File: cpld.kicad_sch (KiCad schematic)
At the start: 1 part, among them U6 ATF1508AS-10AU100

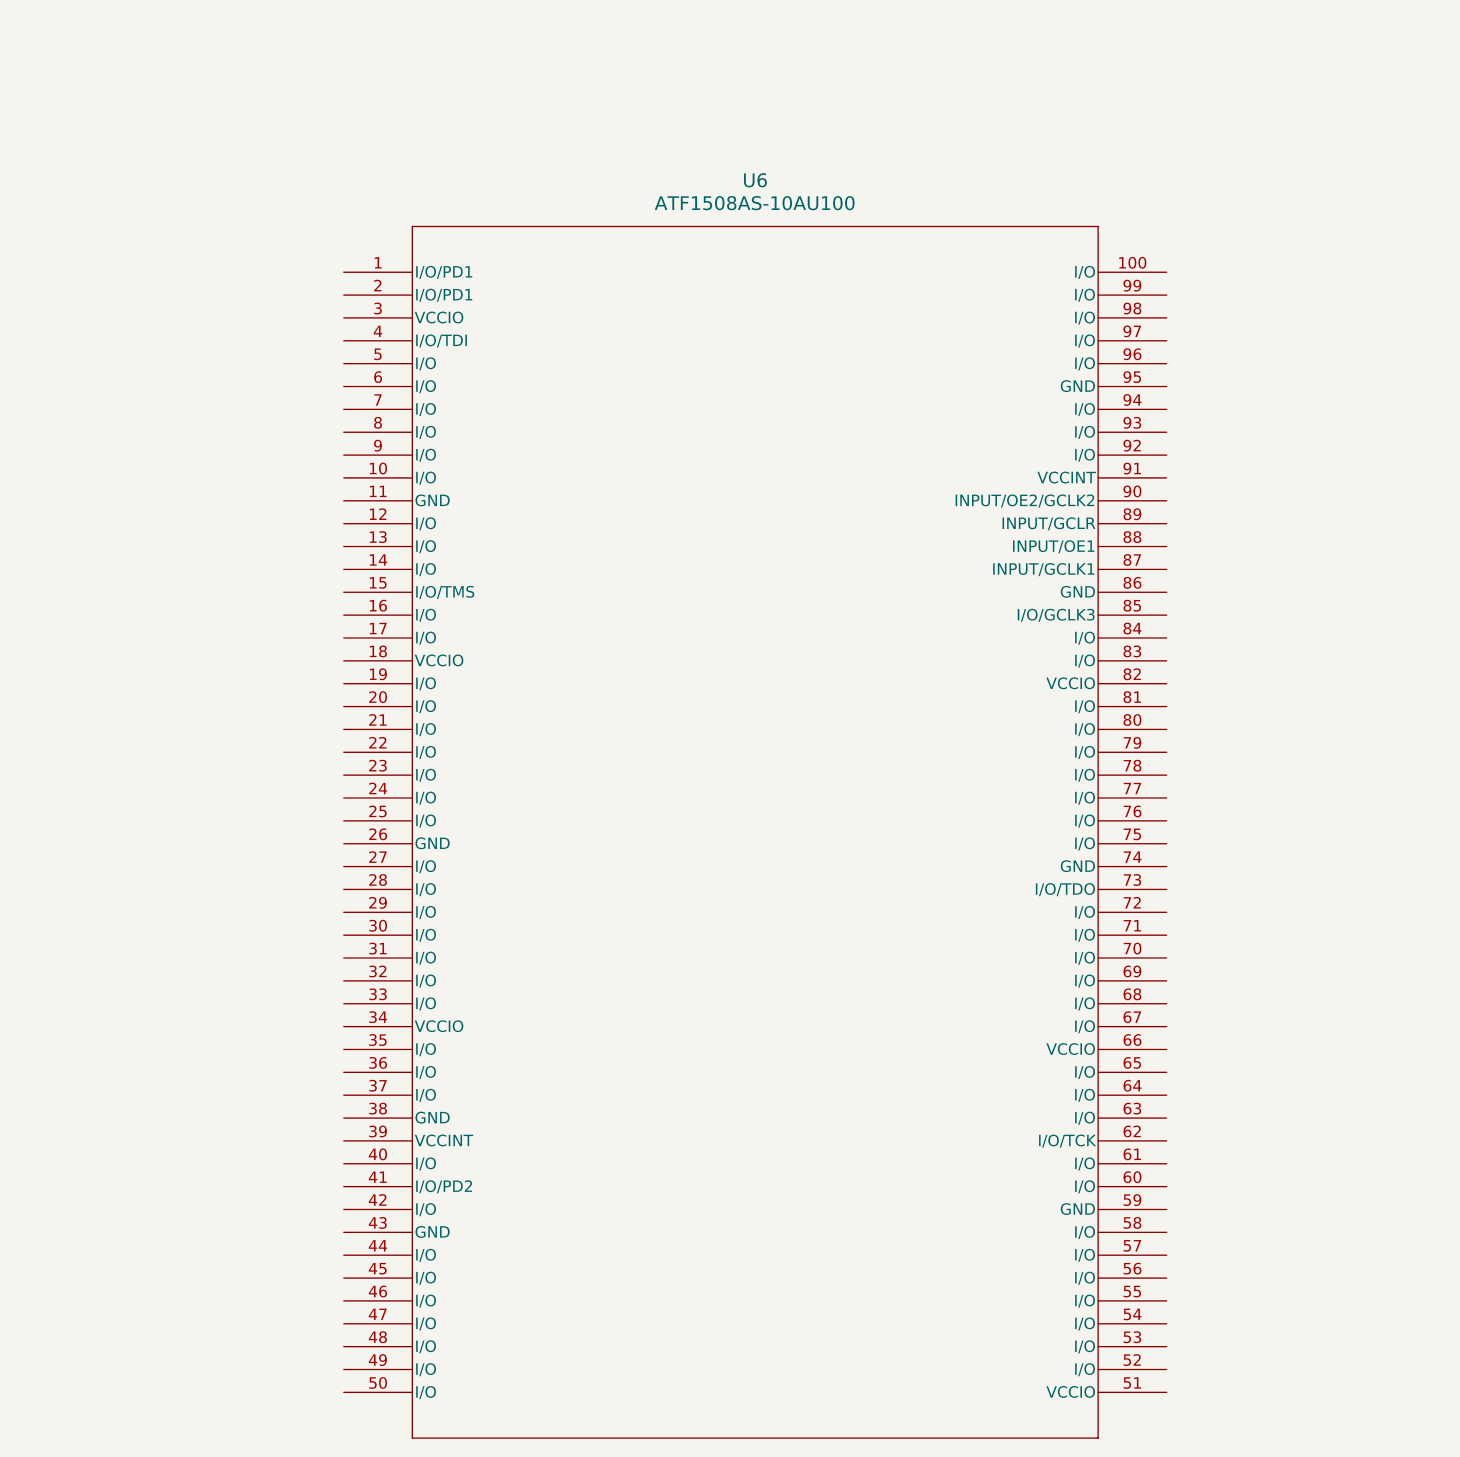
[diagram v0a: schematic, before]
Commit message: Update design
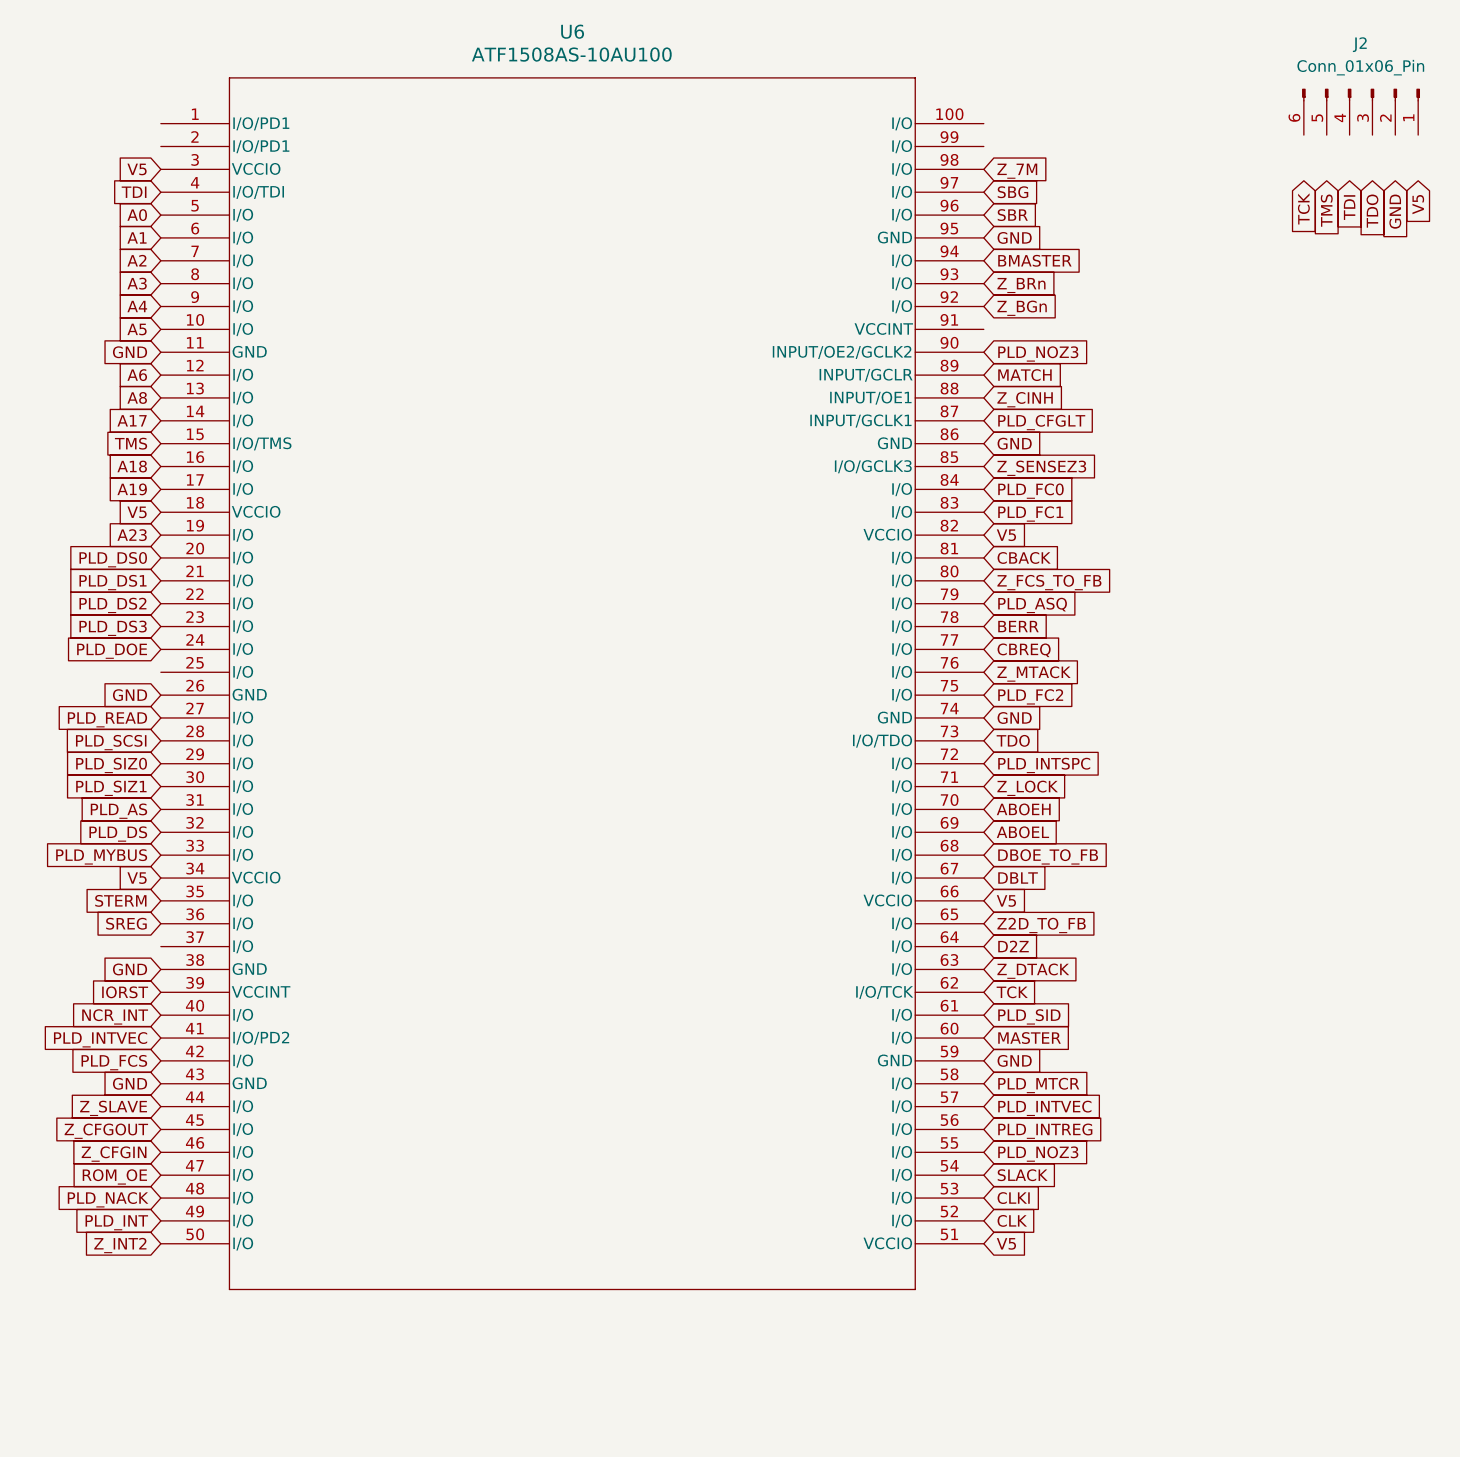
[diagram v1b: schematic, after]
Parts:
- added J2: Conn_01x06_Pin, symbol Connector:Conn_01x06_Pin
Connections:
- net A5: now reaches U6.10 (I/O)
- net GND: now reaches U6.11 (GND)
- net GND: now also U6.26 (GND), U6.38 (GND), U6.43 (GND), U6.59 (GND), U6.74 (GND), U6.86 (GND), U6.95 (GND)
- net A6: now reaches U6.12 (I/O)
- net A8: now reaches U6.13 (I/O)
- net A17: now reaches U6.14 (I/O)
- net TMS: now reaches U6.15 (I/O/TMS)
- net A18: now reaches U6.16 (I/O)
- net A19: now reaches U6.17 (I/O)
- net V5: now reaches U6.18 (VCCIO)
- net V5: now also U6.3 (VCCIO), U6.34 (VCCIO), U6.51 (VCCIO), U6.66 (VCCIO), U6.82 (VCCIO)
- net A23: now reaches U6.19 (I/O)
- net PLD_DS0: now reaches U6.20 (I/O)
- net PLD_DS1: now reaches U6.21 (I/O)
- net PLD_DS2: now reaches U6.22 (I/O)
- net PLD_DS3: now reaches U6.23 (I/O)
- net PLD_DOE: now reaches U6.24 (I/O)
- net PLD_READ: now reaches U6.27 (I/O)
- net PLD_SCSI: now reaches U6.28 (I/O)
- net PLD_SIZ0: now reaches U6.29 (I/O)
- net PLD_SIZ1: now reaches U6.30 (I/O)
- net PLD_AS: now reaches U6.31 (I/O)
- net PLD_DS: now reaches U6.32 (I/O)
- net PLD_MYBUS: now reaches U6.33 (I/O)
- net STERM: now reaches U6.35 (I/O)
- net SREG: now reaches U6.36 (I/O)
- net IORST: now reaches U6.39 (VCCINT)
- net TDI: now reaches U6.4 (I/O/TDI)
- net NCR_INT: now reaches U6.40 (I/O)
- net PLD_INTVEC: now reaches U6.41 (I/O/PD2)
- net PLD_INTVEC: now also U6.57 (I/O)
- net PLD_FCS: now reaches U6.42 (I/O)
- net Z_SLAVE: now reaches U6.44 (I/O)
- net Z_CFGOUT: now reaches U6.45 (I/O)
- net Z_CFGIN: now reaches U6.46 (I/O)
- net ROM_OE: now reaches U6.47 (I/O)
- net PLD_NACK: now reaches U6.48 (I/O)
- net PLD_INT: now reaches U6.49 (I/O)
- net A0: now reaches U6.5 (I/O)
- net Z_INT2: now reaches U6.50 (I/O)
- net CLK: now reaches U6.52 (I/O)
- net CLKI: now reaches U6.53 (I/O)
- net SLACK: now reaches U6.54 (I/O)
- net PLD_NOZ3: now reaches U6.55 (I/O)
- net PLD_NOZ3: now also U6.90 (INPUT/OE2/GCLK2)
- net PLD_INTREG: now reaches U6.56 (I/O)
- net PLD_MTCR: now reaches U6.58 (I/O)
- net A1: now reaches U6.6 (I/O)
- net MASTER: now reaches U6.60 (I/O)
- net PLD_SID: now reaches U6.61 (I/O)
- net TCK: now reaches U6.62 (I/O/TCK)
- net Z_DTACK: now reaches U6.63 (I/O)
- net D2Z: now reaches U6.64 (I/O)
- net Z2D_TO_FB: now reaches U6.65 (I/O)
- net DBLT: now reaches U6.67 (I/O)
- net DBOE_TO_FB: now reaches U6.68 (I/O)
- net ABOEL: now reaches U6.69 (I/O)
- net A2: now reaches U6.7 (I/O)
- net ABOEH: now reaches U6.70 (I/O)
- net Z_LOCK: now reaches U6.71 (I/O)
- net PLD_INTSPC: now reaches U6.72 (I/O)
- net TDO: now reaches U6.73 (I/O/TDO)
- net PLD_FC2: now reaches U6.75 (I/O)
- net Z_MTACK: now reaches U6.76 (I/O)
- net CBREQ: now reaches U6.77 (I/O)
- net BERR: now reaches U6.78 (I/O)
- net PLD_ASQ: now reaches U6.79 (I/O)
- net A3: now reaches U6.8 (I/O)
- net Z_FCS_TO_FB: now reaches U6.80 (I/O)
- net CBACK: now reaches U6.81 (I/O)
- net PLD_FC1: now reaches U6.83 (I/O)
- net PLD_FC0: now reaches U6.84 (I/O)
- net Z_SENSEZ3: now reaches U6.85 (I/O/GCLK3)
- net PLD_CFGLT: now reaches U6.87 (INPUT/GCLK1)
- net Z_CINH: now reaches U6.88 (INPUT/OE1)
- net MATCH: now reaches U6.89 (INPUT/GCLR)
- net A4: now reaches U6.9 (I/O)
- net Z_BGn: now reaches U6.92 (I/O)
- net Z_BRn: now reaches U6.93 (I/O)
- net BMASTER: now reaches U6.94 (I/O)
- net SBR: now reaches U6.96 (I/O)
- net SBG: now reaches U6.97 (I/O)
- net Z_7M: now reaches U6.98 (I/O)
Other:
- moved on the sheet: U6
